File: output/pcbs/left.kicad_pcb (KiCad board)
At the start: 2 copper layers, 130.3 x 118.5 mm, 80 parts

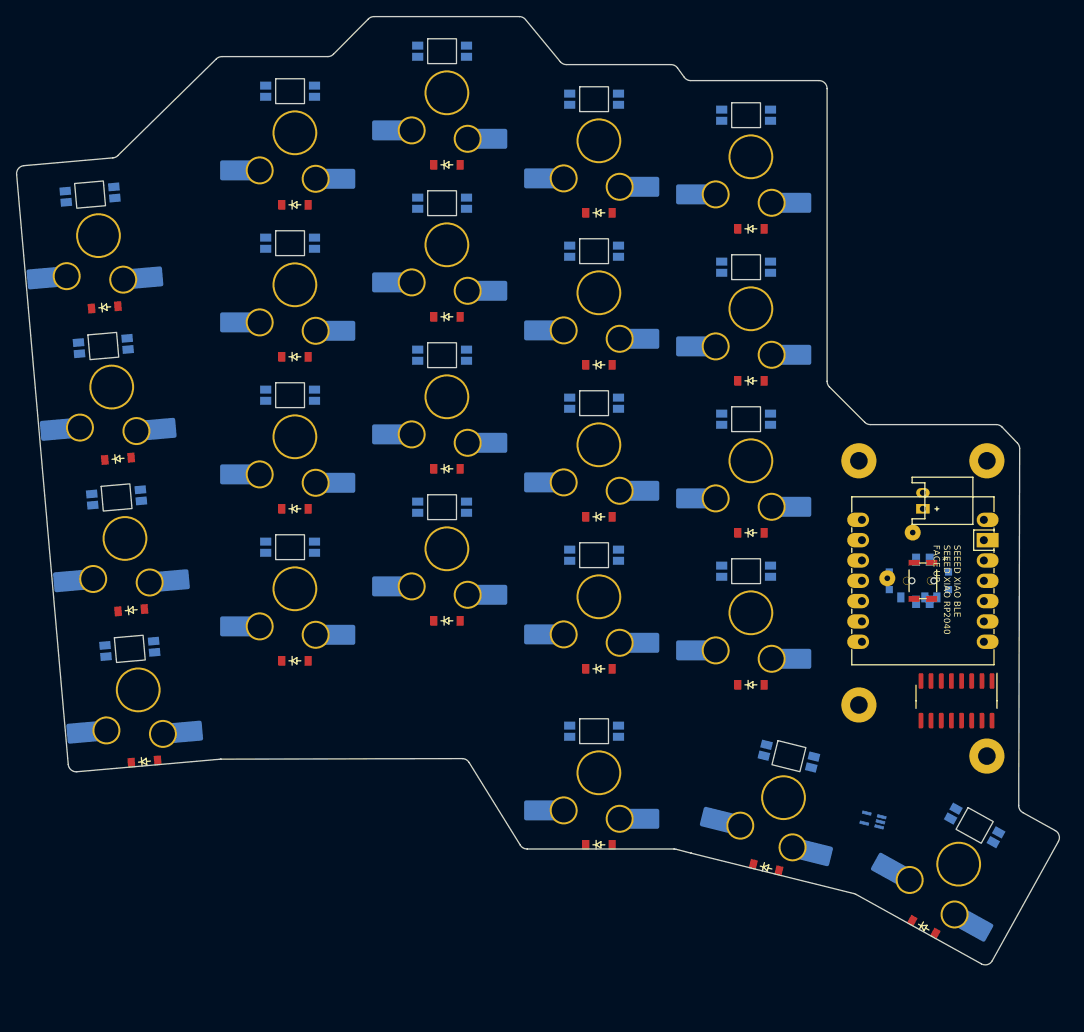
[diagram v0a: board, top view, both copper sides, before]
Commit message: changed pinky layout a bit, almost there!!
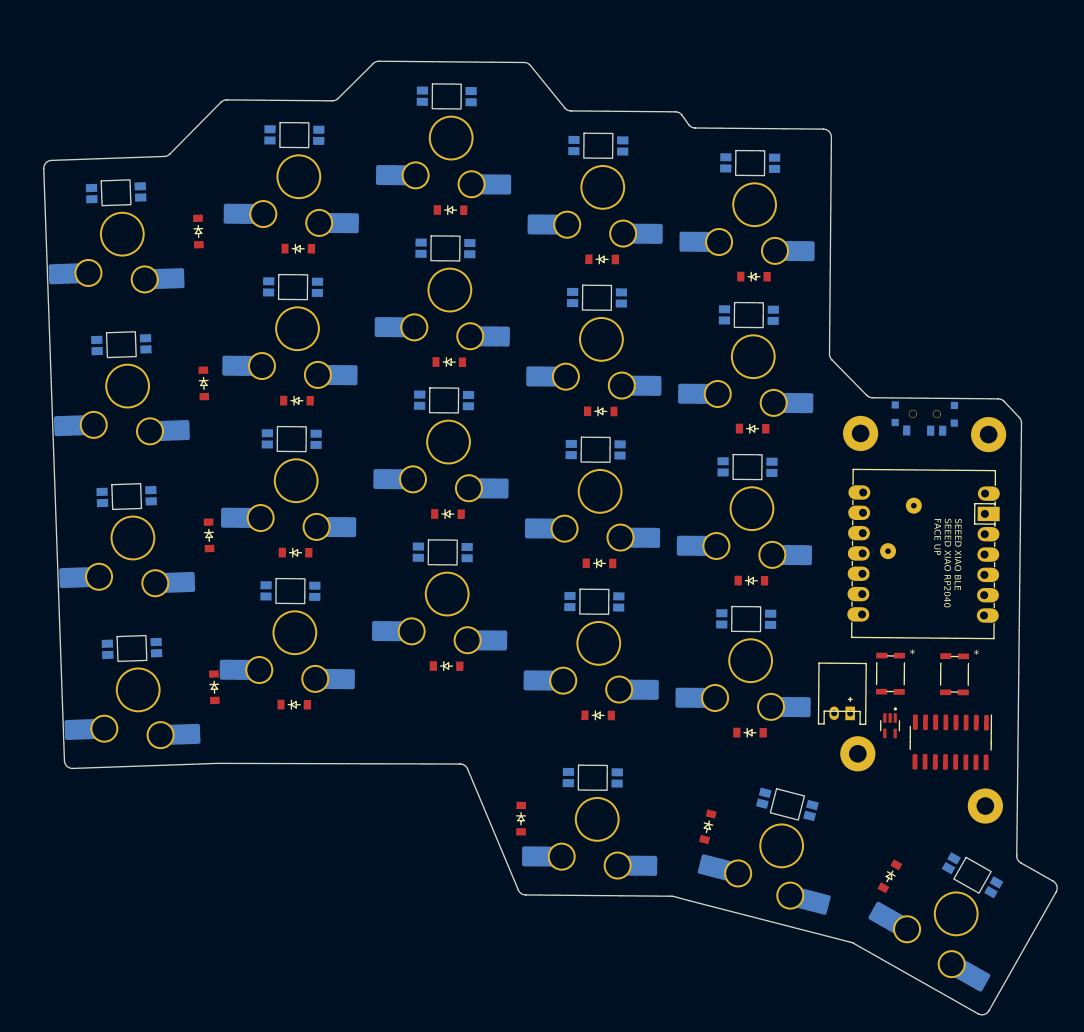
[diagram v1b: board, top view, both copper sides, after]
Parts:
- removed B1: , Panasonic_EVQPUL_EVQPUC
- added _3: SMD_025816_WRE, SMD_025816_WRE, F.Cu at (202.0, 98.0)
- _1: moved to F.Cu
- moved D23 125.6 mm to (107.5, 42.7), turned to -88 degrees
- moved D22 92.8 mm to (108.2, 61.7), turned to -88 degrees
- moved D20 88.2 mm to (109.5, 99.7), turned to -88 degrees
- moved D19 64.3 mm to (194.0, 123.3), turned to -119.5 degrees
- moved D21 62.2 mm to (108.9, 80.7), turned to -88 degrees
- moved D18 37.1 mm to (171.2, 117.1), turned to -104.5 degrees
- moved D17 33.3 mm to (147.9, 116.1), turned to -90.5 degrees
- moved JST1 28.4 mm to (188.0, 102.9), turned to 179.5 degrees
- moved D4 25.3 mm to (120.0, 44.9), turned to -0.5 degrees
- moved D3 23.5 mm to (119.8, 63.9), turned to -0.5 degrees
- moved D12 22.7 mm to (158.0, 46.2), turned to -0.5 degrees
- moved D11 22.6 mm to (157.8, 65.2), turned to -0.5 degrees
- moved D10 22.4 mm to (157.7, 84.2), turned to -0.5 degrees
- moved D9 22.3 mm to (157.5, 103.2), turned to -0.5 degrees
- moved D2 21.8 mm to (119.7, 82.9), turned to -0.5 degrees
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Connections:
- D1 pad 2: pinky_bottom -> ring_bottom
- D10 pad 2: middle_home -> index_home
- D11 pad 2: middle_top -> index_top
- D12 pad 2: middle_number -> index_number
- D13 pad 2: index_bottom -> inner_bottom
- D14 pad 2: index_home -> inner_home
- D15 pad 2: index_top -> inner_top
- D16 pad 2: index_number -> inner_number
- D17 pad 1: Row0 -> Row4
- D17 pad 2: inner_bottom -> near_thumb
- D18 pad 1: Row1 -> Row4
- D18 pad 2: inner_home -> home_thumb
- D19 pad 1: Row2 -> Row4
- D19 pad 2: inner_top -> far_thumb
- D2 pad 2: pinky_home -> ring_home
- D20 pad 1: Row3 -> Row0
- D20 pad 2: inner_number -> pinky_bottom
- D21 pad 1: Row4 -> Row1
- D21 pad 2: near_thumb -> pinky_home
- D22 pad 1: Row4 -> Row2
- D22 pad 2: home_thumb -> pinky_top
- D23 pad 1: Row4 -> Row3
- D23 pad 2: far_thumb -> pinky_number
- D3 pad 2: pinky_top -> ring_top
- D4 pad 2: pinky_number -> ring_number
- D5 pad 2: ring_bottom -> middle_bottom
- D6 pad 2: ring_home -> middle_home
- D7 pad 2: ring_top -> middle_top
- D8 pad 2: ring_number -> middle_number
- D9 pad 2: middle_bottom -> index_bottom
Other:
- board size 130.3 x 118.5 mm -> 126.7 x 119.2 mm

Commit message: close to finishing layout/placement
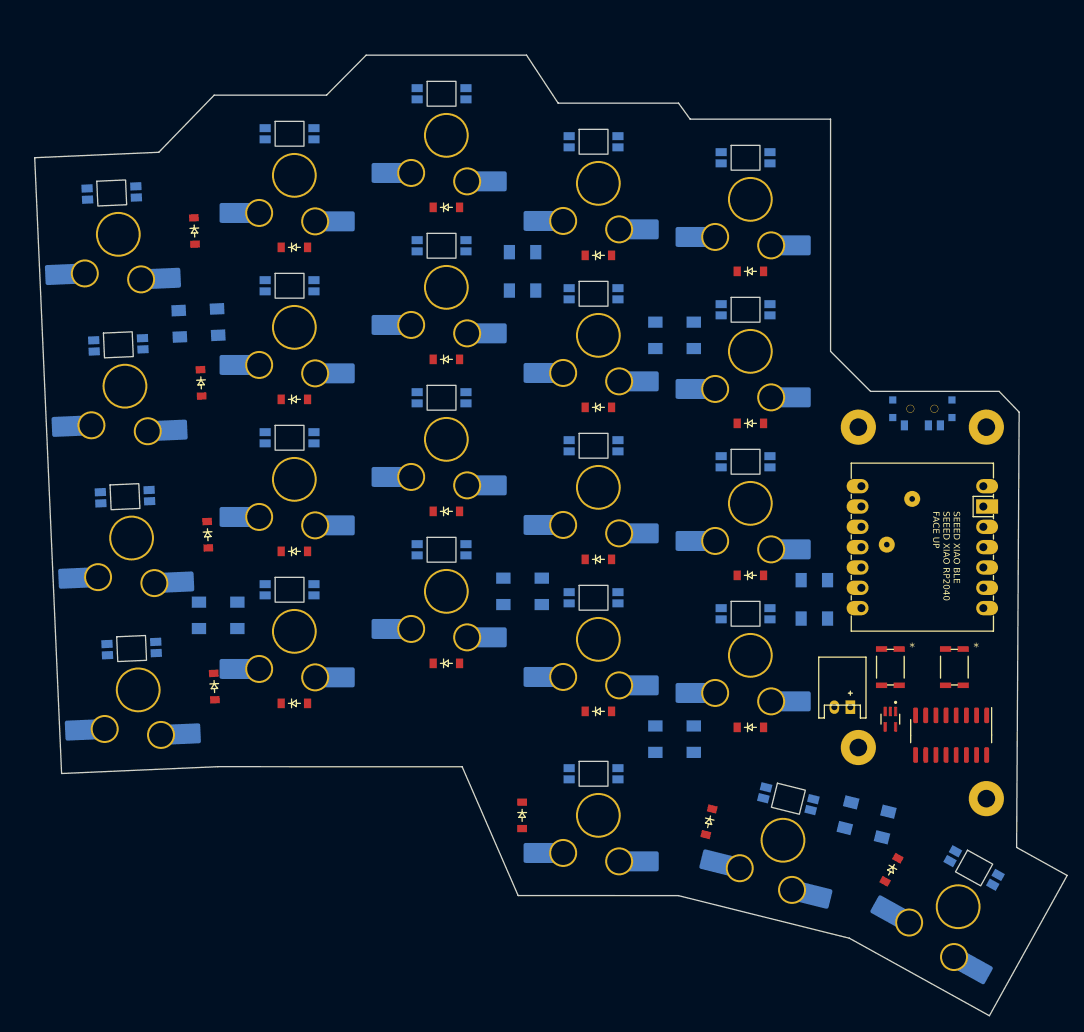
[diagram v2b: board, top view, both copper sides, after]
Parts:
- added LED24: VAL**, WS2812B, B.Cu at (107.5, 54.1)
- added LED25: VAL**, WS2812B, B.Cu at (110.0, 90.7)
- added LED26: VAL**, WS2812B, B.Cu at (148.0, 87.7)
- added LED27: VAL**, WS2812B, B.Cu at (167.0, 106.2)
- added LED28: VAL**, WS2812B, B.Cu at (191.0, 116.2)
- added LED29: VAL**, WS2812B, B.Cu at (167.0, 55.7)
- added LED30: VAL**, WS2812B, B.Cu at (184.5, 88.7)
- added LED31: VAL**, WS2812B, B.Cu at (148.0, 47.7)
- moved PAD1 0.97 mm to (206.0, 67.2), turned to 0 degrees
- moved PAD3 0.93 mm to (206.0, 113.6), turned to -29 degrees
- moved LED23 0.93 mm to (204.5, 122.3), turned to -29 degrees
- moved S23 0.93 mm to (202.5, 127.1), turned to -29 degrees
- moved _3 0.89 mm to (202.0, 97.2), turned to -90 degrees
- moved 19.051 0.89 mm to (201.6, 105.7), turned to -90 degrees
- moved LED20 0.88 mm to (175.9, 33.5), turned to 0 degrees
- moved MCU1 0.87 mm to (198.0, 82.2), turned to 0 degrees
- moved S20 0.86 mm to (176.5, 38.7), turned to 0 degrees
- moved D19 0.84 mm to (194.2, 122.5), turned to -119 degrees
- moved PAD2 0.84 mm to (190.0, 67.2), turned to 0 degrees
- moved _1 0.82 mm to (194.0, 103.7), turned to -90 degrees
- moved _2 0.82 mm to (194.0, 97.2), turned to -90 degrees
- moved D16 0.81 mm to (176.5, 47.7), turned to 0 degrees
- moved PAD4 0.79 mm to (190.0, 107.2), turned to -14 degrees
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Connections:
- LED4 pad 2: LEDEND -> LED_BACKLIGHT_1
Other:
- board size 126.7 x 119.2 mm -> 129.1 x 120.1 mm
